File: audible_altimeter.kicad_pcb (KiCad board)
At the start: 2 copper layers, 52 x 29 mm, 54 parts, among them CON1 BUQ2-USB-MICRO-B, IC1 BUQ2-ATXMEGA128A4U-A, P1 CONN_2, P2 SERIAL, Q1 NPN-SOT23, U1 MCP7940M, U10 CNT, U11 DWN, U12 2SMPB-01-01, U13 FLASH_MEMORY, U14 MCP4017, U2 MCP73831-SOT-23-5, U3 NCP4681-SC-70, U4 UP, U5 MPL3115A2, U6 MS5805-02BA01, U7 LS013B4DN04, U8 SPEAKER-WITH-DUMMY, U9 TAG-CONNECT-ATMEL-PDI-CONNECT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, X1 CRYSTAL

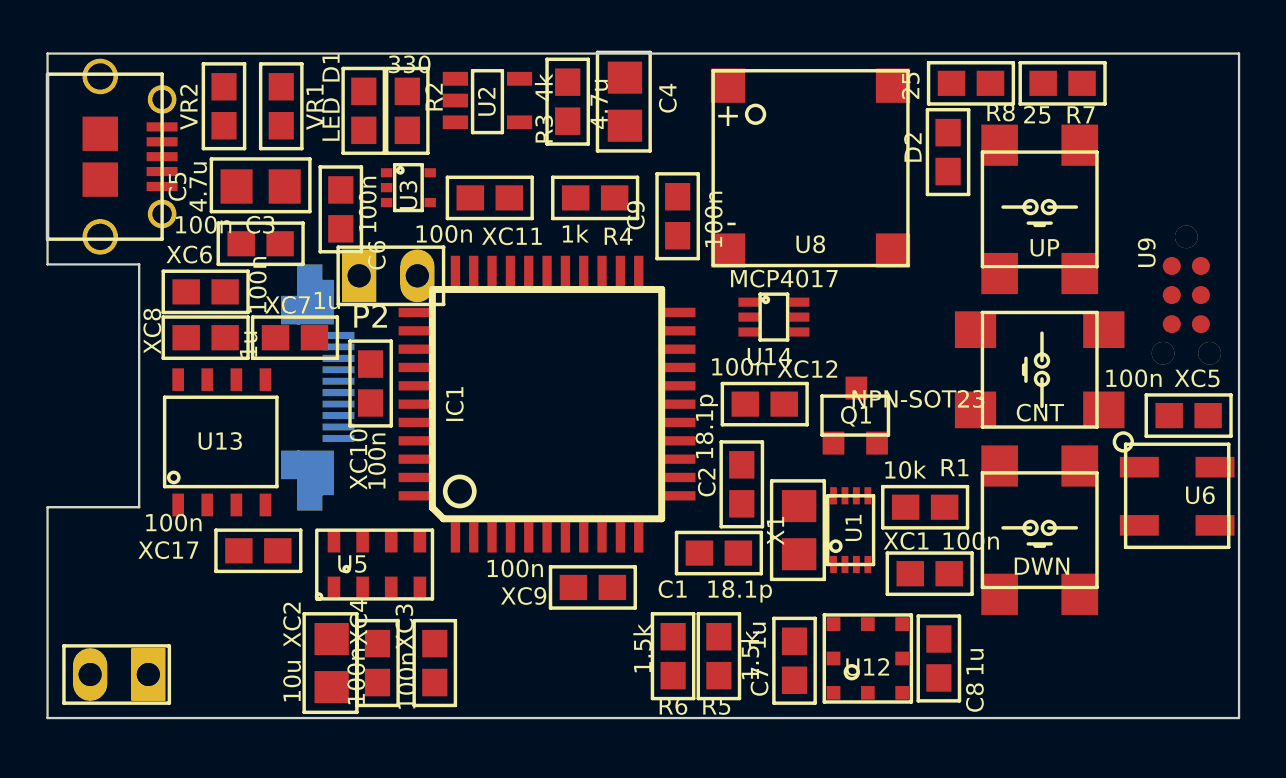
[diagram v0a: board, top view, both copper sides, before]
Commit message: Before starting laying out tracks
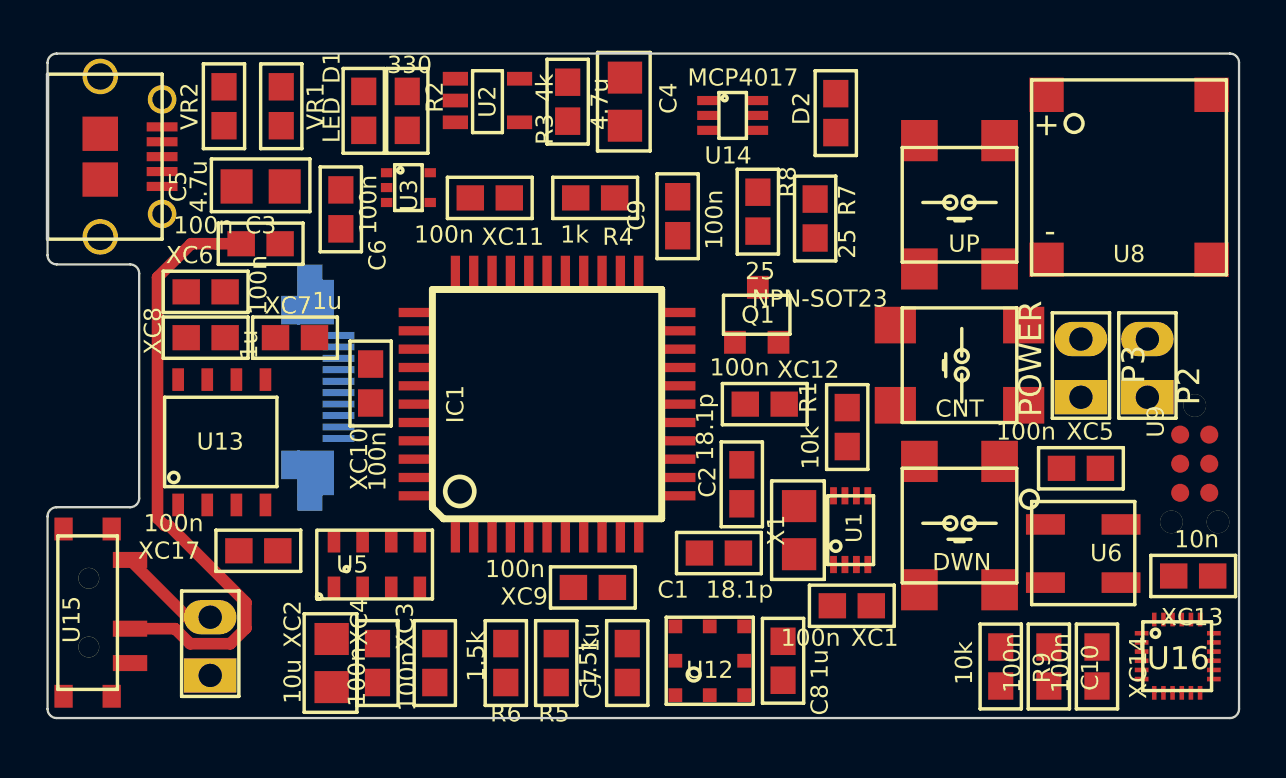
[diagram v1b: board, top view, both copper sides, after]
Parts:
- added C10: 100n, buq2:SM0603, F.Cu at (179.4, 123.0)
- added P3: POWER, buq2:PIN_HEADER_2, F.Cu at (180.8, 111.2)
- added R9: 10k, buq2:SM0603, F.Cu at (177.3, 123.0)
- added U15: SPDT-SWITCH, buq2:CUS-12TB-SWITCH, F.Cu at (137.5, 120.6)
- added U16: MPU-9250, buq2:24QFN-3MM-3MM, F.Cu at (183.5, 121.5)
- added XC13: 10n, buq2:SM0603, F.Cu at (185.7, 119.0)
- added XC14: 100n, buq2:SM0603, F.Cu at (181.5, 123.0)
- moved P2 34.8 mm to (183.7, 111.2), turned to 90 degrees
- moved U8 13.9 mm to (182.9, 101.6)
- moved R7 12.3 mm to (169.2, 103.4), turned to 90 degrees
- moved R8 10.9 mm to (166.7, 103.1), turned to 90 degrees
- moved U14 8.98 mm to (165.6, 98.9)
- moved U9 7.37 mm to (185.8, 111.6)
- moved R6 7.31 mm to (155.7, 122.8)
- moved C7 7.30 mm to (161.0, 122.8)
- moved R5 7.11 mm to (157.9, 122.8)
- moved U12 6.90 mm to (164.6, 122.7)
- moved C8 6.80 mm to (167.8, 122.7)
- moved Q1 6.15 mm to (166.7, 107.6)
- moved XC5 5.23 mm to (180.8, 114.3)
- moved D2 5.19 mm to (170.1, 98.8)
- moved R1 4.88 mm to (170.6, 112.5), turned to 90 degrees
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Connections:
- net /Barometer/I2C_SCL renamed /Accelerometer/I2C_SCL
- net /Barometer/I2C_SDA renamed /Accelerometer/I2C_SDA
- IC1 pad 24: (no net) -> /Buzzer/BUZZER_DRIVE
- IC1 pad 40: (no net) -> /Battery/+3.3V
- IC1 pad 5: (no net) -> /MCU/ACC_INT
- P1 pad 2: /Battery/BATTERY -> /Battery/BATTERY-DIRECT
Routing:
- net /Battery/BATTERY: track 0.00 -> 26.9 mm
- net /Battery/BATTERY-DIRECT: track 0.00 -> 4.54 mm
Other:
- outline, holes or cut-outs redrawn
- board text added: "AudibleA V3.0 Matti Jukola 2015-04-17"
- board text removed: "AudibleA V2.0 Matti Jukola 2015-01-27"
